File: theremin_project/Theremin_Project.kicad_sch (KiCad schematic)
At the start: 25 parts, among them J1 USB_C_Receptacle, U1 AD8001AR, U2 HEF4093B, U3 AD8001AR, U4 ESP32-S2-SOLO-N4R2, U8 NCP164CSN330T1G

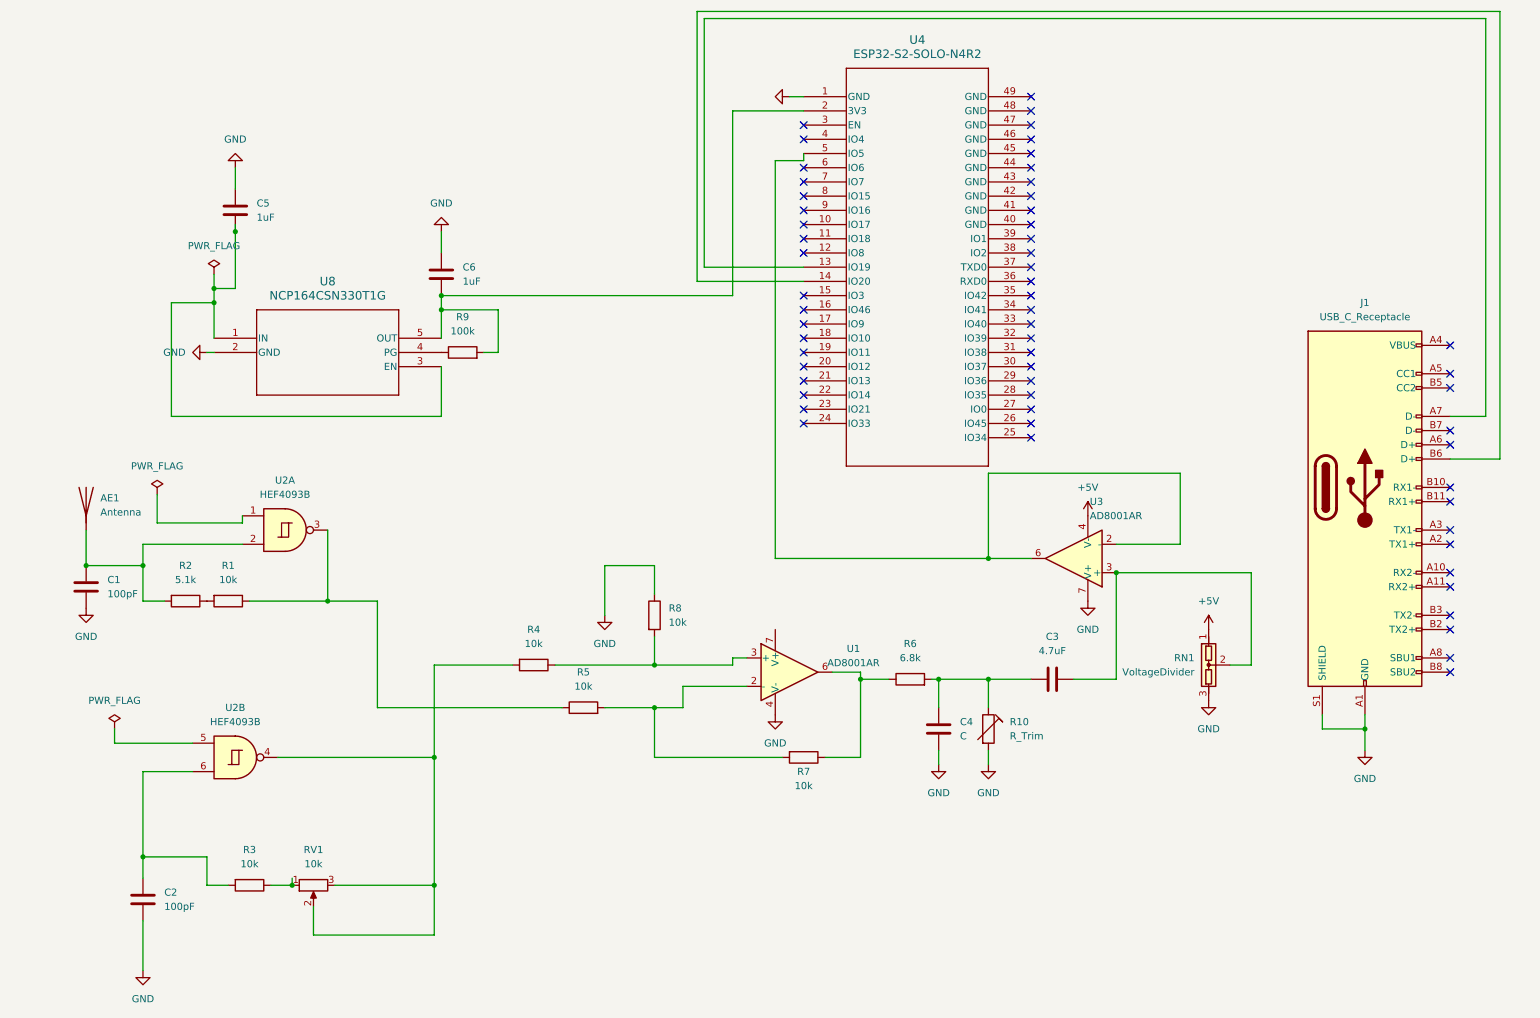
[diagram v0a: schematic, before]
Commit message: layout and sch
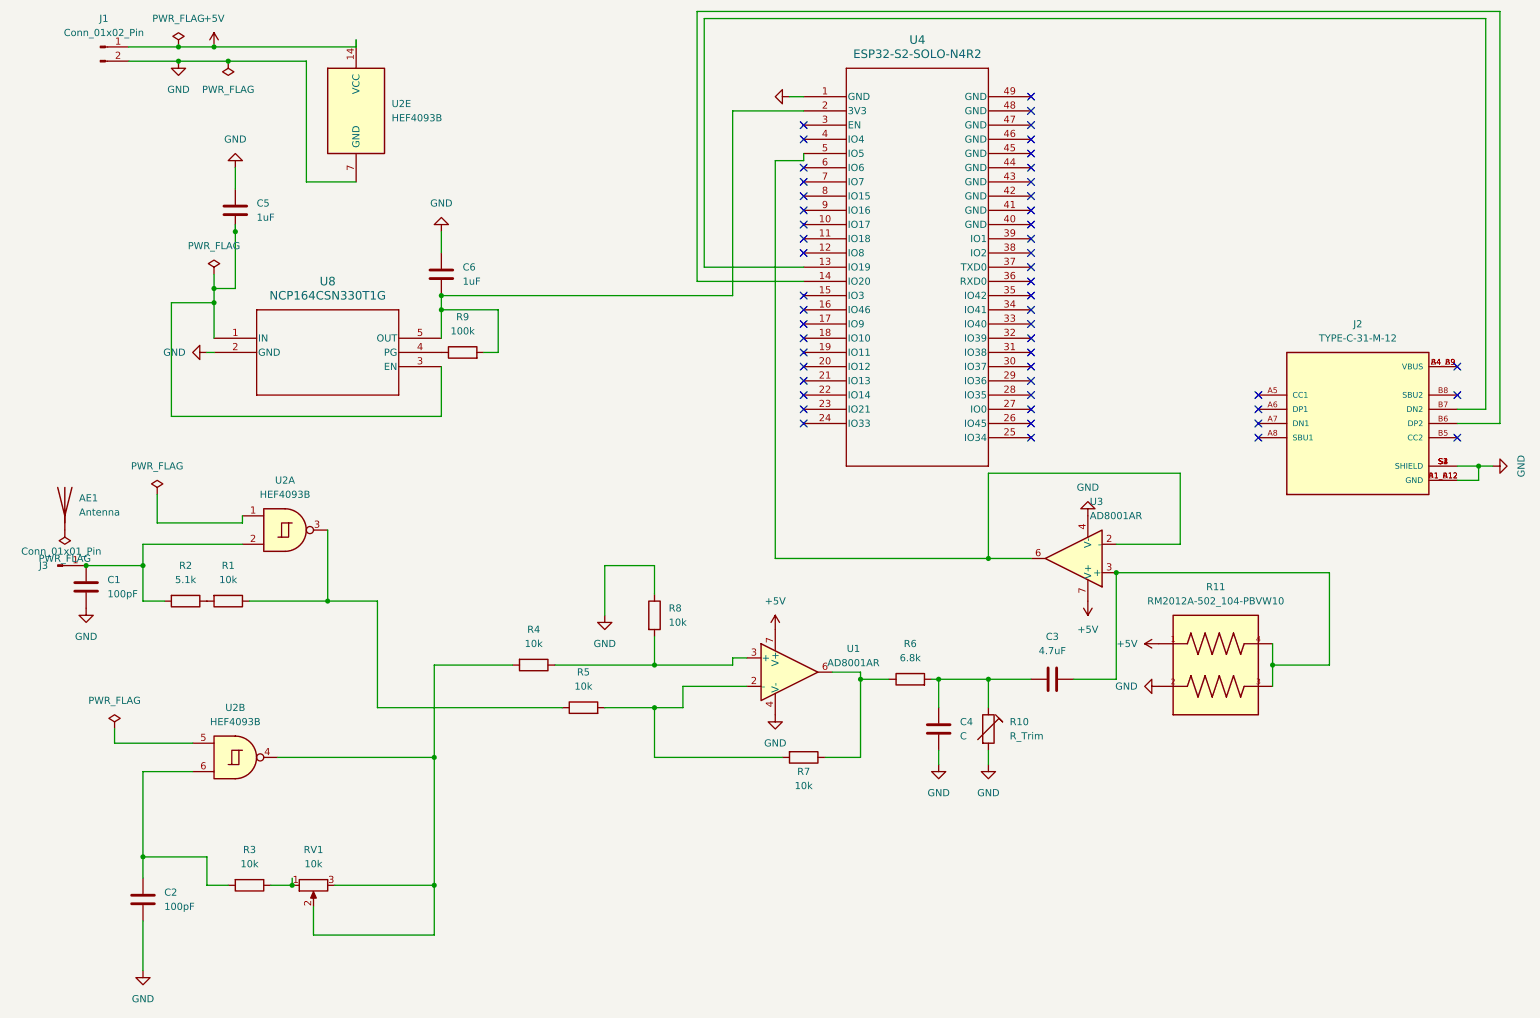
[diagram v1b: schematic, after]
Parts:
- removed J1: USB_C_Receptacle, symbol Connector:USB_C_Receptacle
- removed RN1: VoltageDivider, symbol Device:VoltageDivider
- added J1: Conn_01x02_Pin, Connector_PinHeader_2.54mm:PinHeader_1x02_P2.54mm_Vertical, symbol Connector:Conn_01x02_Pin
- added J2: TYPE-C-31-M-12, TYPE-C-31-M-12:HRO_TYPE-C-31-M-12, symbol TYPE-C-31-M-12:TYPE-C-31-M-12
- added J3: Conn_01x01_Pin, Connector_PinHeader_1.00mm:PinHeader_1x01_P1.00mm_Vertical, symbol Connector:Conn_01x01_Pin
- added R11: RM2012A-502_104-PBVW10, RM2012A-502_104-PBVW10:RESCAXE_RM2012-4N, symbol RM2012A-502_104-PBVW10:RM2012A-502_104-PBVW10
- added unit 5 of U2
- R9: footprint (none) -> Resistor_THT:R_Axial_DIN0204_L3.6mm_D1.6mm_P1.90mm_Vertical
- U2: footprint (none) -> HEF4093BP_652:DIP254P762X420-14
- U4: footprint MOD41_ESP32-S2-SOLO_EXP -> esp32:MOD41_ESP32-S2-SOLO_EXP; symbol 2024-04-04_02-12-16:ESP32-S2-SOLO-N4R2 -> esp32:ESP32-S2-SOLO-N4R2
- U8: footprint FP-NCP164CSN330T1G_OSI -> NCP:FP-NCP164CSN330T1G_OSI; symbol linreg:NCP164CSN330T1G -> ncp:NCP164CSN330T1G
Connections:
- net +5V: now also U1.7 (V+), U3.7 (V+), J1.1 (Pin_1), R11.1, U2.14 (VCC); no longer U3.4 (V-)
- net GND: now also U3.4 (V-), J1.2 (Pin_2), J2.A1_B12 (GND), J2.B1_A12 (GND), J2.S1 (SHIELD), J2.S2 (SHIELD), J2.S3 (SHIELD), J2.S4 (SHIELD), R11.2, U2.7 (GND); no longer U3.7 (V+)
- net at C1.1, R2.2, U2.2: now also J3.1 (Pin_1); no longer AE1.1 (A)
- net at U4.13 (IO19): now also J2.B7 (DN2)
- net at U4.14 (IO20): now also J2.B6 (DP2)
- net at C3.1, U3.3 (+): now also R11.3, R11.4
- new net: J2.A4_B9 (VBUS), J2.B4_A9 (VBUS)
- no-connect marks 59 -> 51
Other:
- moved on the sheet: AE1
